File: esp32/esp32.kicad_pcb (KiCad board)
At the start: 2 copper layers, 1 part, among them U1 ESP32-DEVKITC-32U

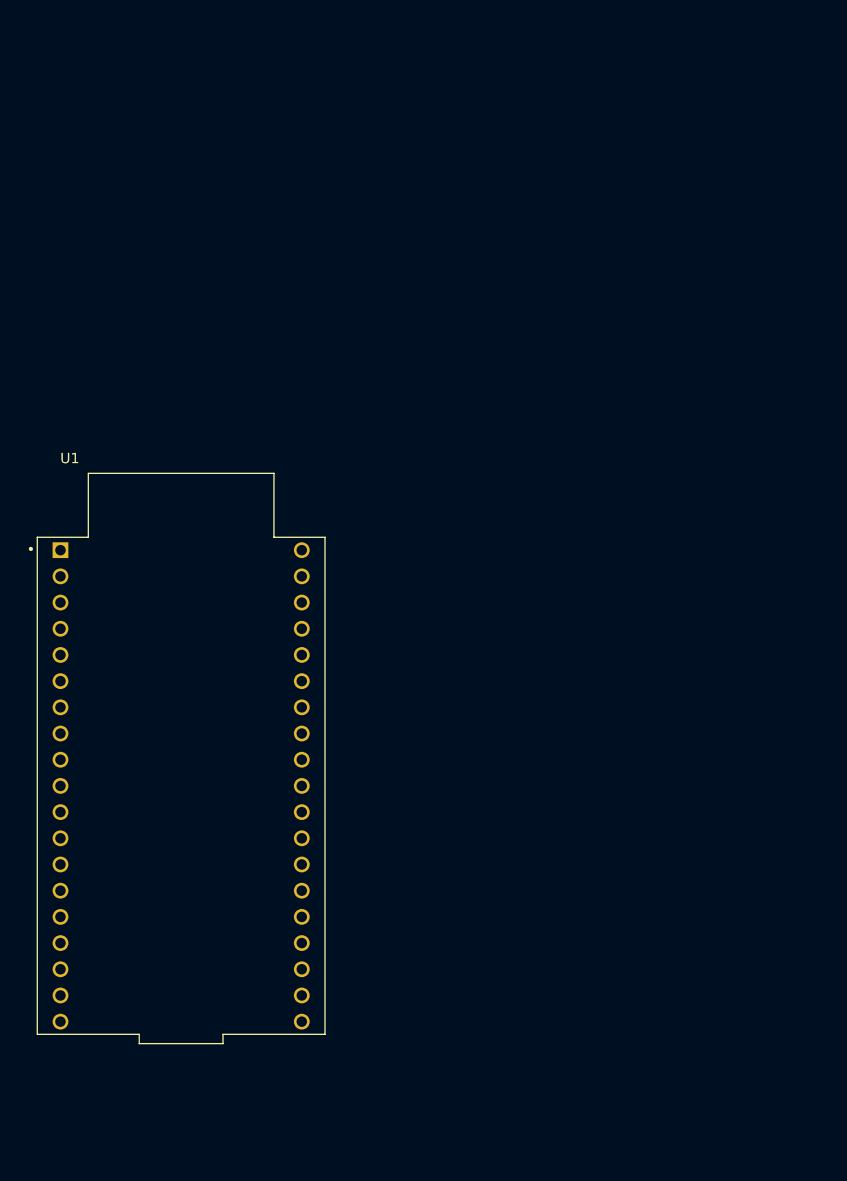
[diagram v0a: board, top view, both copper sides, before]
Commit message: esp32
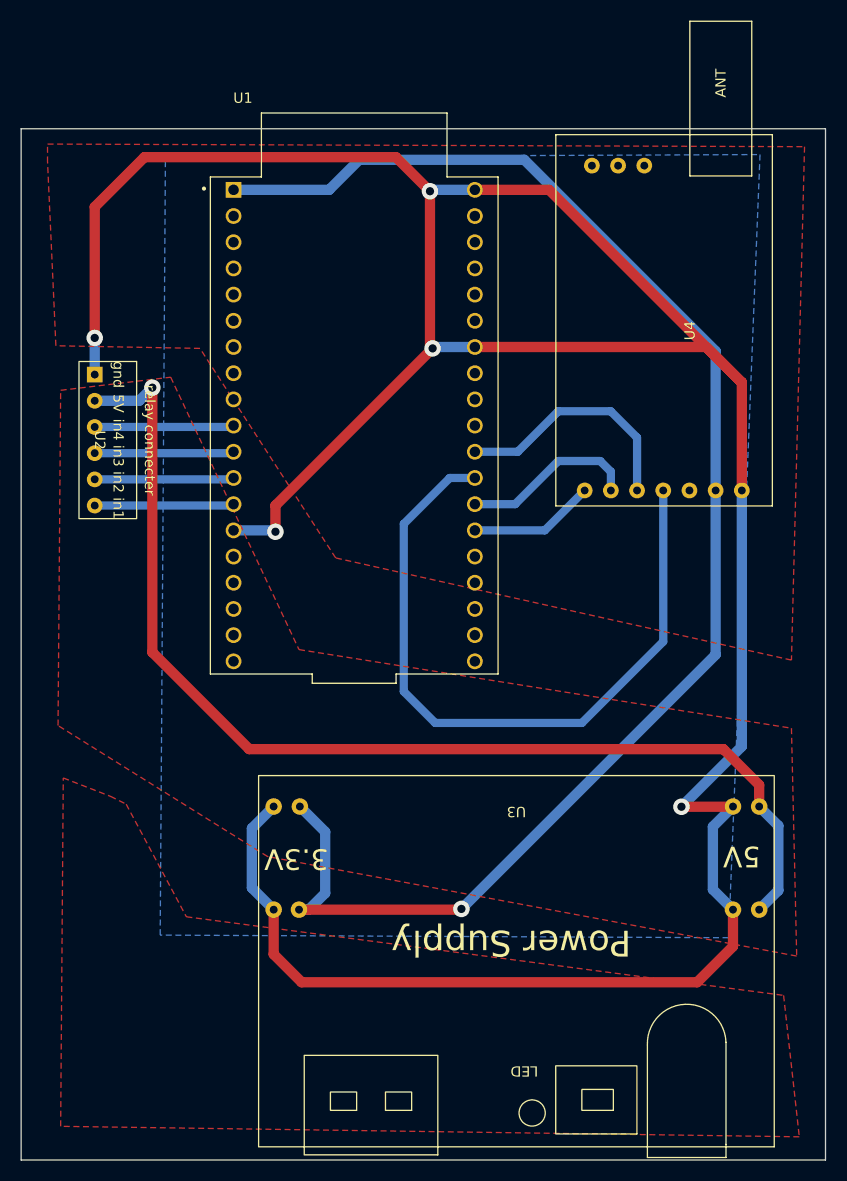
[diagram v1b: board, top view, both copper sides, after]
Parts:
- added U2: relay_4_out, module_analog_sensor:relay_4_out, F.Cu at (132.3, 73.9)
- added U3: asm1117_3.3v_5v, module_analog_sensor:asm1117_3.3V_5V, F.Cu at (173.2, 109.5)
- added U4: E32-433T20D, 42CrMo4-KiCad-Library:E32-xxxT20D, F.Cu at (177.0, 80.3)
- moved U1 38.8 mm to (157.5, 72.5)
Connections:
- U1 pad 1: unconnected-(U1-Pad1) -> +3.3V
- U1 pad 10: unconnected-(U1-Pad10) -> Net-(U1-Pad10)
- U1 pad 11: unconnected-(U1-Pad11) -> Net-(U1-Pad11)
- U1 pad 12: unconnected-(U1-Pad12) -> Net-(U1-Pad12)
- U1 pad 13: unconnected-(U1-Pad13) -> Net-(U1-Pad13)
- U1 pad 14: unconnected-(U1-Pad14) -> GND
- U1 pad 25: unconnected-(U1-Pad25) -> Net-(U1-Pad25)
- U1 pad 26: unconnected-(U1-Pad26) -> Net-(U1-Pad26)
- U1 pad 27: unconnected-(U1-Pad27) -> Net-(U1-Pad27)
- U1 pad 28: unconnected-(U1-Pad28) -> Net-(U1-Pad28)
- U1 pad 32: unconnected-(U1-Pad32) -> GND
- U1 pad 38: unconnected-(U1-Pad38) -> GND
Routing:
- net GND: track 0.00 -> 292.3 mm, vias 0 -> 5
- net +3.3V: track 0.00 -> 148.3 mm, vias 0 -> 1
- net +5V: track 0.00 -> 109.6 mm, vias 0 -> 1
- net Net-(U1-Pad27): track 0.00 -> 69.3 mm
- net Net-(U1-Pad28): track 0.00 -> 23.5 mm
- net Net-(U1-Pad26): track 0.00 -> 17.2 mm
- net Net-(U1-Pad13): track 0.00 -> 13.5 mm
- net Net-(U1-Pad12): track 0.00 -> 13.5 mm
- net Net-(U1-Pad11): track 0.00 -> 13.5 mm
- net Net-(U1-Pad10): track 0.00 -> 13.5 mm
- net Net-(U1-Pad25): track 0.00 -> 12.3 mm
- added copper zone on B.Cu, net +3.3V
- added copper zone on F.Cu, net +5V
- added copper zone on F.Cu, net GND
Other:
- board outline added: 78 x 100 mm
